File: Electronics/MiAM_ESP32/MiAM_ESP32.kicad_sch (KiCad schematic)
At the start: 17 parts, among them J1 Conn_01x06_Male, J10 Conn_01x03_Male, J14 Conn_01x02_Male, J2 Conn_01x06_Male, J3 Screw_Terminal_01x02, J6 Conn_01x04_Male, J7 Conn_01x02_Male, J9 Conn_01x03_Male, U1 ESP32-DEVKIT-V1, U2 3V3, U3 MT3608, U4 TB6612FNG, U5 LM7805_TO220

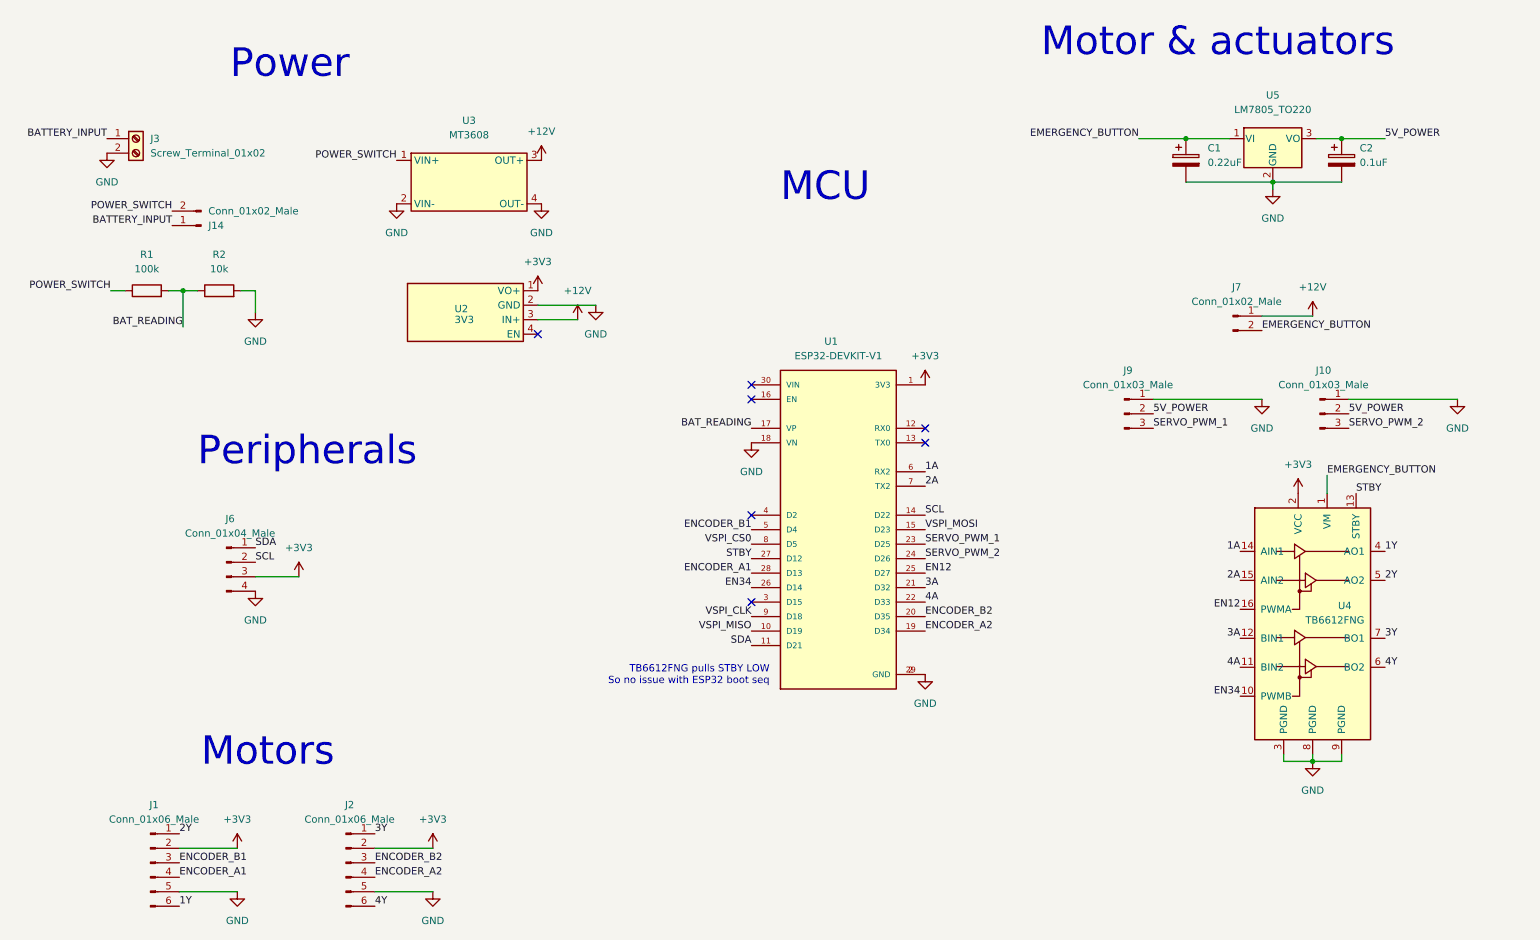
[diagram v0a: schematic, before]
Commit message: Fix initial PAMI pcb
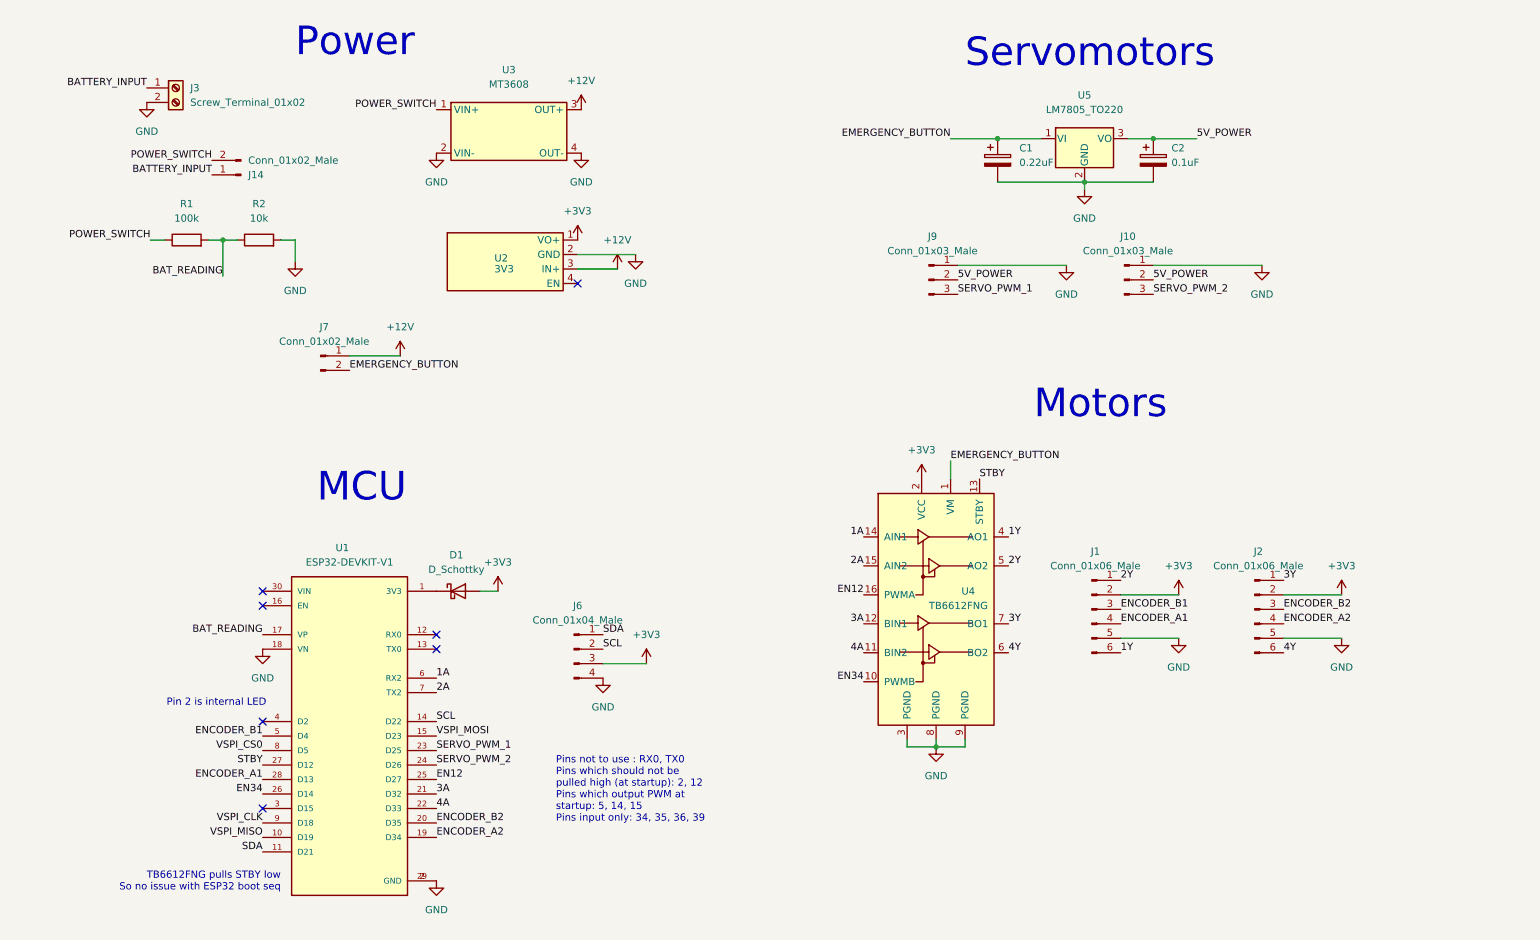
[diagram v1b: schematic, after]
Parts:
- added D1: D_Schottky, Diode_THT:D_DO-41_SOD81_P7.62mm_Horizontal, symbol Device:D_Schottky
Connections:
- net +3V3: now also D1.2 (A); no longer U1.1 (3V3)
- new net: D1.1 (K), U1.1 (3V3)
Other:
- note added: "Pin 2 is internal LED"
- note added: "Pins not to use : RX0, TX0 Pins which should not be pulled high (at startup): 2, 12 Pins which output PWM at startup: 5, 14, 15 Pins input only: 34, 35, 36, 39"
- note added: "Servomotors"
- note added: "TB6612FNG pulls STBY low So no issue with ESP32 boot seq"
- note removed: "Motor & actuators"
- note removed: "Peripherals"
- note removed: "TB6612FNG pulls STBY LOW So no issue with ESP32 boot seq"
- moved on the sheet: C1, C2, J1, J10, J14, J2, J3, J6, J7, J9, R1, R2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
